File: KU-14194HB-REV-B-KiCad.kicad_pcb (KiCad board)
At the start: 2 copper layers, 387.7 x 180.3 mm, 92 parts, among them CN1 KEYBOARD_20PIN_MALE, CN10 LED_CONNECTOR, CN2 USER_PORT_CON, CN3 CASSETTE_PORT_CON, CN4 SERIAL_BUS_CON, CN7 POWER_CON, CN8 CONTROL_PORT, CN9 CONTROL_PORT, Q1 2SC1815, Q2 2SC1815, Q3 TP298/2SD880, SW1 POWER_SWITCH, U1 CIA_U1, U2 CIA_U2, U20 556, U27 7408_U27, U28 4066_U28, U7 6510_MPU, U8 7406N

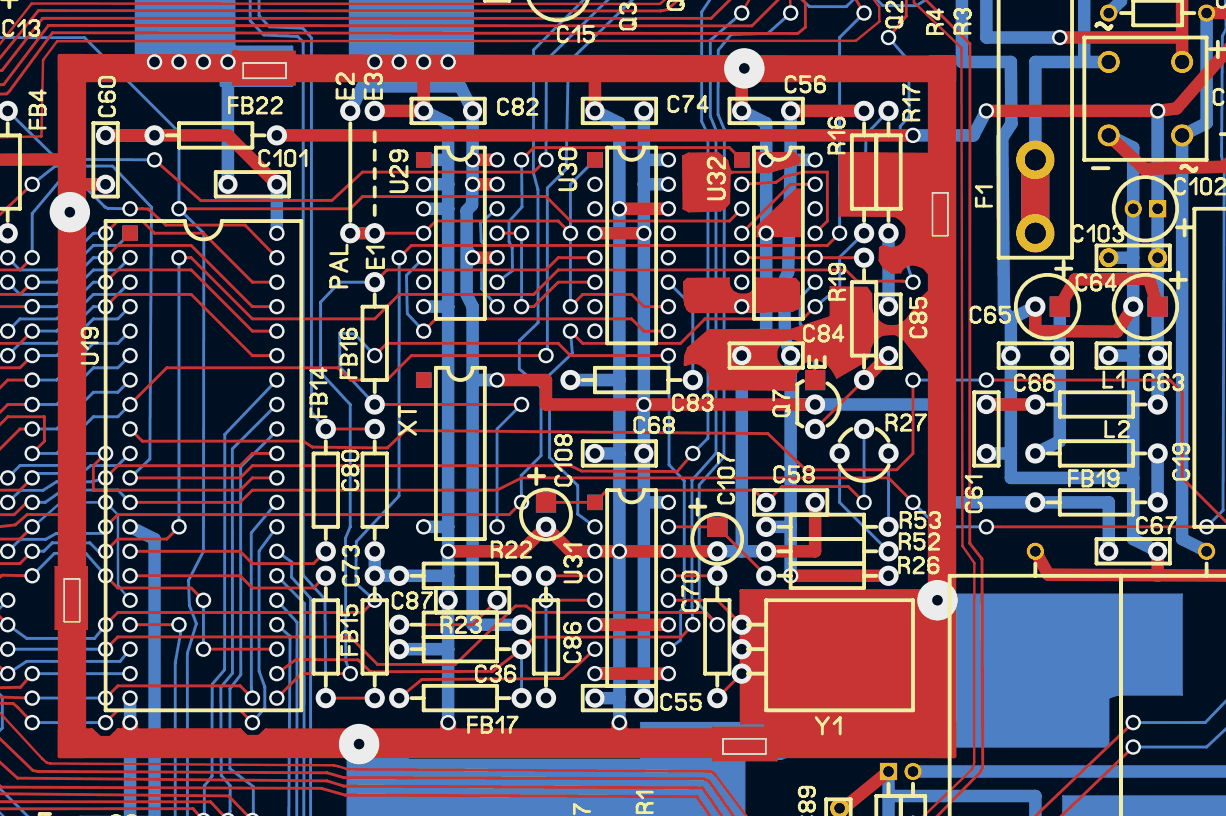
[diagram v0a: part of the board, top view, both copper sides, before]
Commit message: Oscillator area
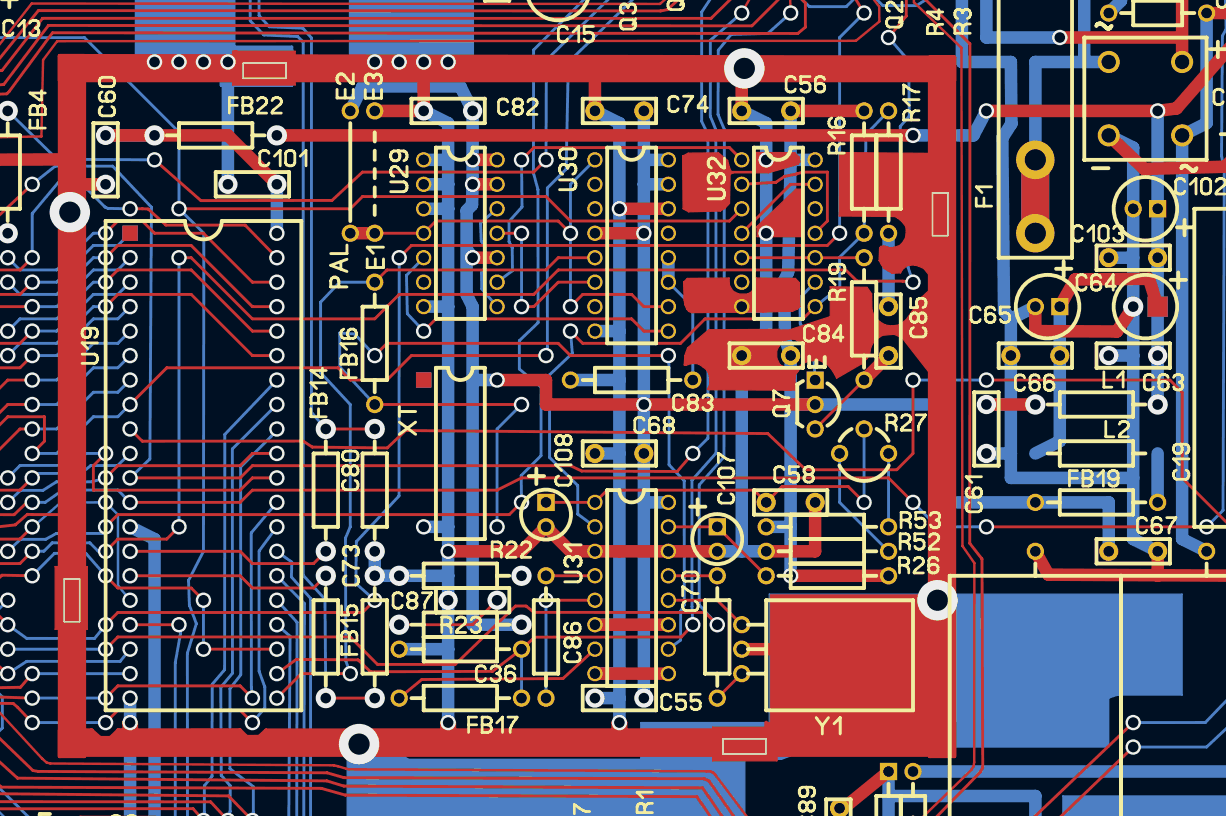
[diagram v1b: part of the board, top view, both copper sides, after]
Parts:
- added C107: 10uF, KU-14194HB-RevB-KiCad:CAP_ELYT_RADIAL_P2.54mm, F.Cu at (317.5, 167.6)
- added C108: 10uF, KU-14194HB-RevB-KiCad:CAP_ELYT_RADIAL_P2.54mm, F.Cu at (299.7, 165.1)
- added C36: .1, KU-14194HB-RevB-KiCad:RESISTOR, F.Cu at (297.2, 180.3)
- added C56: .1, KU-14194HB-RevB-KiCad:CAP_P5.08mm, F.Cu at (325.1, 124.5)
- added C58: .1, KU-14194HB-RevB-KiCad:CAP_P5.08mm, F.Cu at (322.6, 165.1)
- added C65: 10uF, KU-14194HB-RevB-KiCad:CAP_ELYT_RADIAL_P2.54mm, F.Cu at (353.1, 144.8)
- added C66: .1, KU-14194HB-RevB-KiCad:CAP_P5.08mm, F.Cu at (353.1, 149.9)
- added C67: .1, KU-14194HB-RevB-KiCad:CAP_P5.08mm, F.Cu at (358.1, 170.2)
- added C68: .1, KU-14194HB-RevB-KiCad:CAP_P5.08mm, F.Cu at (309.9, 160.0)
- added C70: ~, KU-14194HB-RevB-KiCad:RESISTOR, F.Cu at (317.5, 185.4)
- added C74: .1, KU-14194HB-RevB-KiCad:CAP_P5.08mm, F.Cu at (309.9, 124.5)
- added C83: 82pF, KU-14194HB-RevB-KiCad:RESISTOR, F.Cu at (315.0, 152.4)
- added C84: .1, KU-14194HB-RevB-KiCad:CAP_P5.08mm, F.Cu at (325.1, 149.9)
- added C85: .47, KU-14194HB-RevB-KiCad:CAP_P5.08mm, F.Cu at (335.3, 144.8)
- added C86: ?, KU-14194HB-RevB-KiCad:RESISTOR, F.Cu at (299.7, 185.4)
- added E1: JUMPER_WIRE, KU-14194HB-RevB-KiCad:JUMPER_WIRE, F.Cu at (279.4, 137.2)
- added FB16: FERRITE_NARROW, KU-14194HB-RevB-KiCad:FERRITE_BEAD_TH_P12.7mm, F.Cu at (281.9, 148.6)
- added FB17: FERRITE_NARROW, KU-14194HB-RevB-KiCad:FERRITE_BEAD_TH_P12.7mm, F.Cu at (290.8, 185.4)
- added FB19: FERRITE_NARROW, KU-14194HB-RevB-KiCad:FERRITE_BEAD_TH_P12.7mm, F.Cu at (356.9, 165.1)
- added Q7: 2SC1815, KU-14194HB-RevB-KiCad:Q_NPN_ECB, F.Cu at (327.7, 154.9)
- added R16: 1K, KU-14194HB-RevB-KiCad:RESISTOR, F.Cu at (332.7, 124.5)
- added R17: 2K7, KU-14194HB-RevB-KiCad:RESISTOR, F.Cu at (335.3, 124.5)
- added R19: 15K, KU-14194HB-RevB-KiCad:RESISTOR, F.Cu at (332.7, 152.4)
- added R26: 100, KU-14194HB-RevB-KiCad:RESISTOR, F.Cu at (335.3, 172.7)
- added R27: 500, KU-14194HB-RevB-KiCad:POTMETER, F.Cu at (332.7, 160.0)
- added R52: ?, KU-14194HB-RevB-KiCad:RESISTOR, F.Cu at (335.3, 170.2)
- added R53: ?, KU-14194HB-RevB-KiCad:RESISTOR, F.Cu at (322.6, 167.6)
- added U29: 74LS74, KU-14194HB-RevB-KiCad:DIP14, F.Cu at (290.8, 137.2)
- added U30: 74LS193, KU-14194HB-RevB-KiCad:DIP16, F.Cu at (308.6, 138.4)
- added U31: 74LS629N, KU-14194HB-RevB-KiCad:DIP16, F.Cu at (308.6, 174.0)
- added U32: MC4044, KU-14194HB-RevB-KiCad:DIP14, F.Cu at (323.9, 137.2)
- added Y1: Crystal, KU-14194HB-RevB-KiCad:CRYSTAL, F.Cu at (320.0, 180.3)
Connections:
- R36 pad 2: Net-(R36-Pad2) -> ~RESET~
- U7 pad 1: Net-(U7-Pad1) -> PHI_0
- U8 pad 12: Net-(R36-Pad2) -> ~RESET~
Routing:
- net /Sheet1/+9V_UNREG: track 1275.8 -> 0.00 mm, vias 49 -> 0
- net Earth: track 4815.6 -> 5978.7 mm, vias 118 -> 136
- net (no net): track 12170.6 -> 11054.7 mm, vias 556 -> 442
- net /Sheet1/+Vc: track 0.00 -> 314.6 mm, vias 0 -> 11
- net PHI_0: track 0.00 -> 270.1 mm, vias 0 -> 4
- net Net-(U7-Pad1): track 270.1 -> 0.00 mm, vias 5 -> 0
- net DOT_CLOCK: track 0.00 -> 148.4 mm, vias 0 -> 4
- net Net-(FB16-Pad1): track 0.00 -> 105.8 mm, vias 0 -> 4
- net PHI_COLOR: track 0.00 -> 79.0 mm, vias 0 -> 2
- net Net-(R16-Pad2): track 0.00 -> 74.5 mm, vias 0 -> 1
- net /Sheet1/jumper_select: track 0.00 -> 51.4 mm, vias 0 -> 2
- net Net-(C108-Pad1): track 0.00 -> 43.1 mm, vias 0 -> 1
- net Net-(U29-Pad9): track 0.00 -> 38.0 mm, vias 0 -> 1
- net Net-(U29-Pad5): track 0.00 -> 35.5 mm, vias 0 -> 1
- net /Sheet1/CAN+5V: track 144.6 -> 175.3 mm
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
